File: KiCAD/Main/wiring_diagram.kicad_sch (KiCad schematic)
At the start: 19 parts, among them J5 Screw_Terminal_01x09, J6 Screw_Terminal_01x09, M1 Motor_Servo [Axon Mini MkII], M2 Motor_Servo [Axon Mini MkII], SW3 Screw Switch, SW4 Screw Switch, SW5 Screw Switch, SW6 Screw Switch

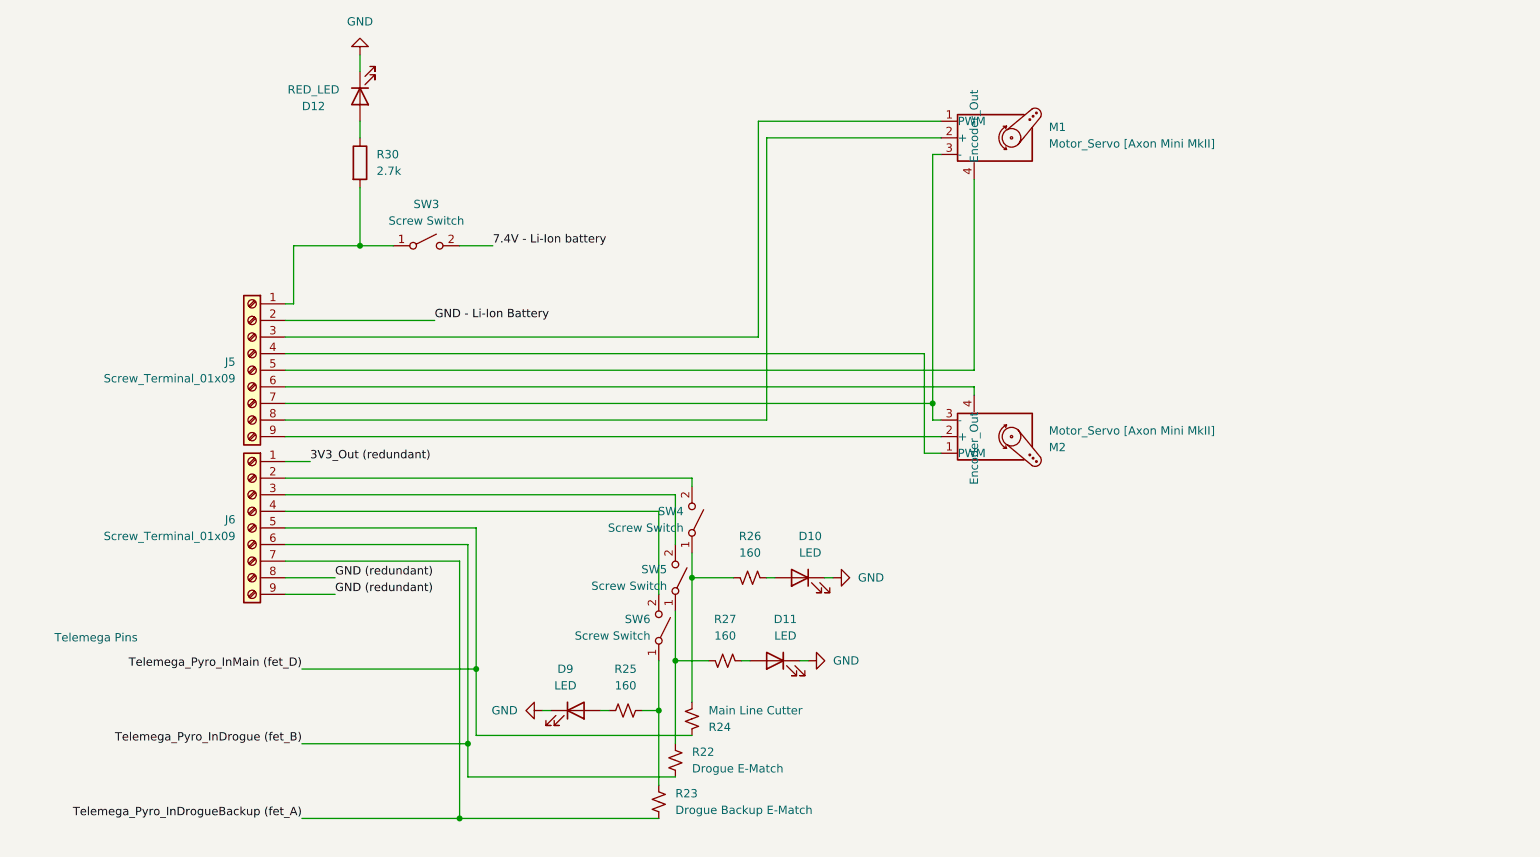
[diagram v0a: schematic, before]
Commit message: Submit design for review
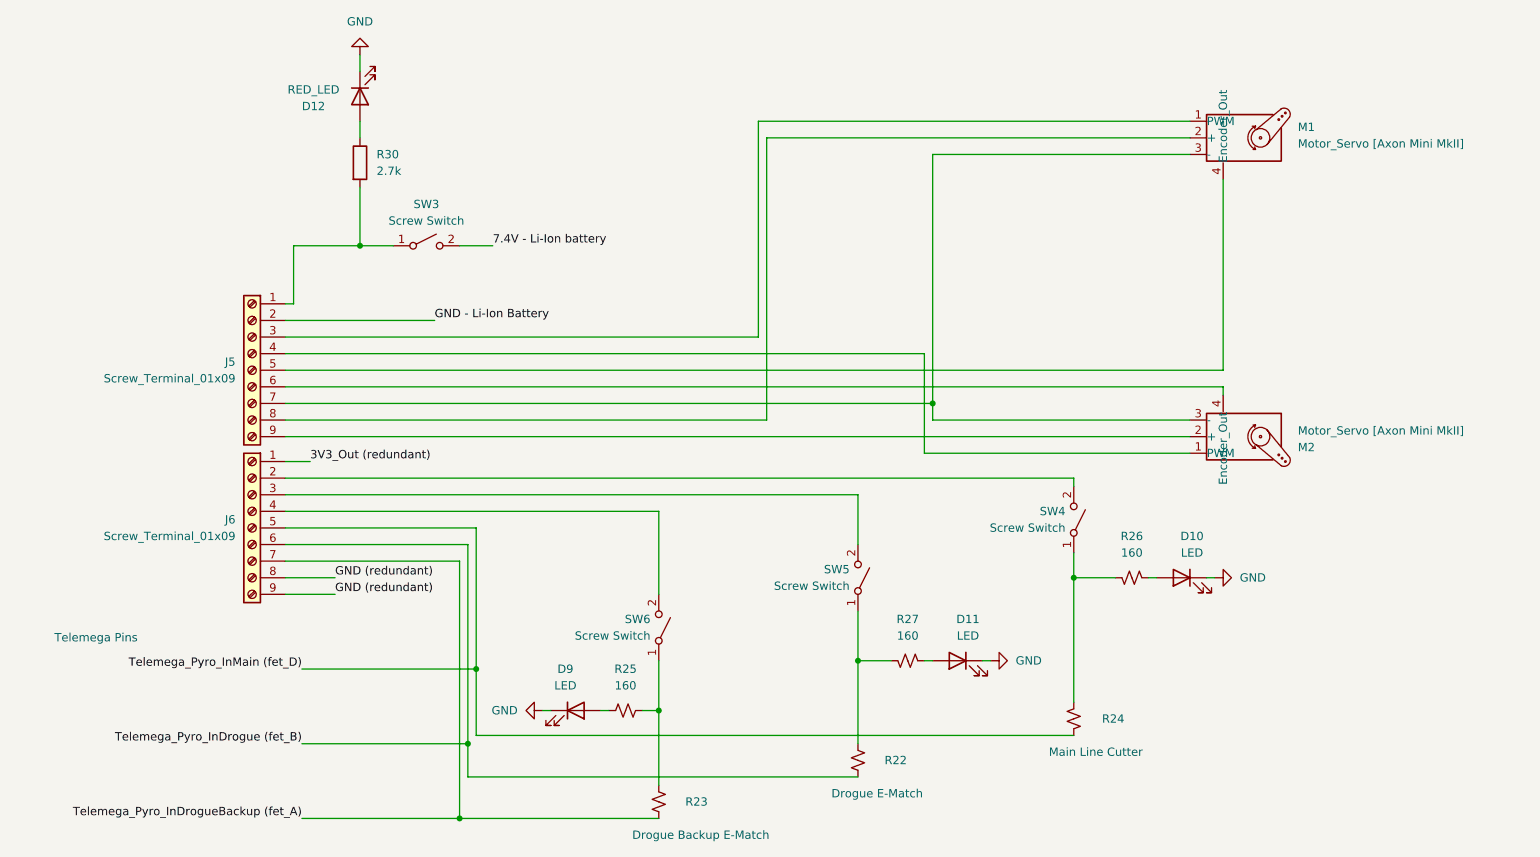
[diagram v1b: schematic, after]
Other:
- moved on the sheet: D10, D11, M1, M2, R22, R24, R26, R27, SW4, SW5
